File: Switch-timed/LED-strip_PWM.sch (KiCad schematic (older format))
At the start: 17 parts, among them IC1 MADW__ATTINY13-MM, P1 CONN_2, P2 CONN_2, T1 AO3400, U1 MCP6001, U2 MCP1804-SOT23-5

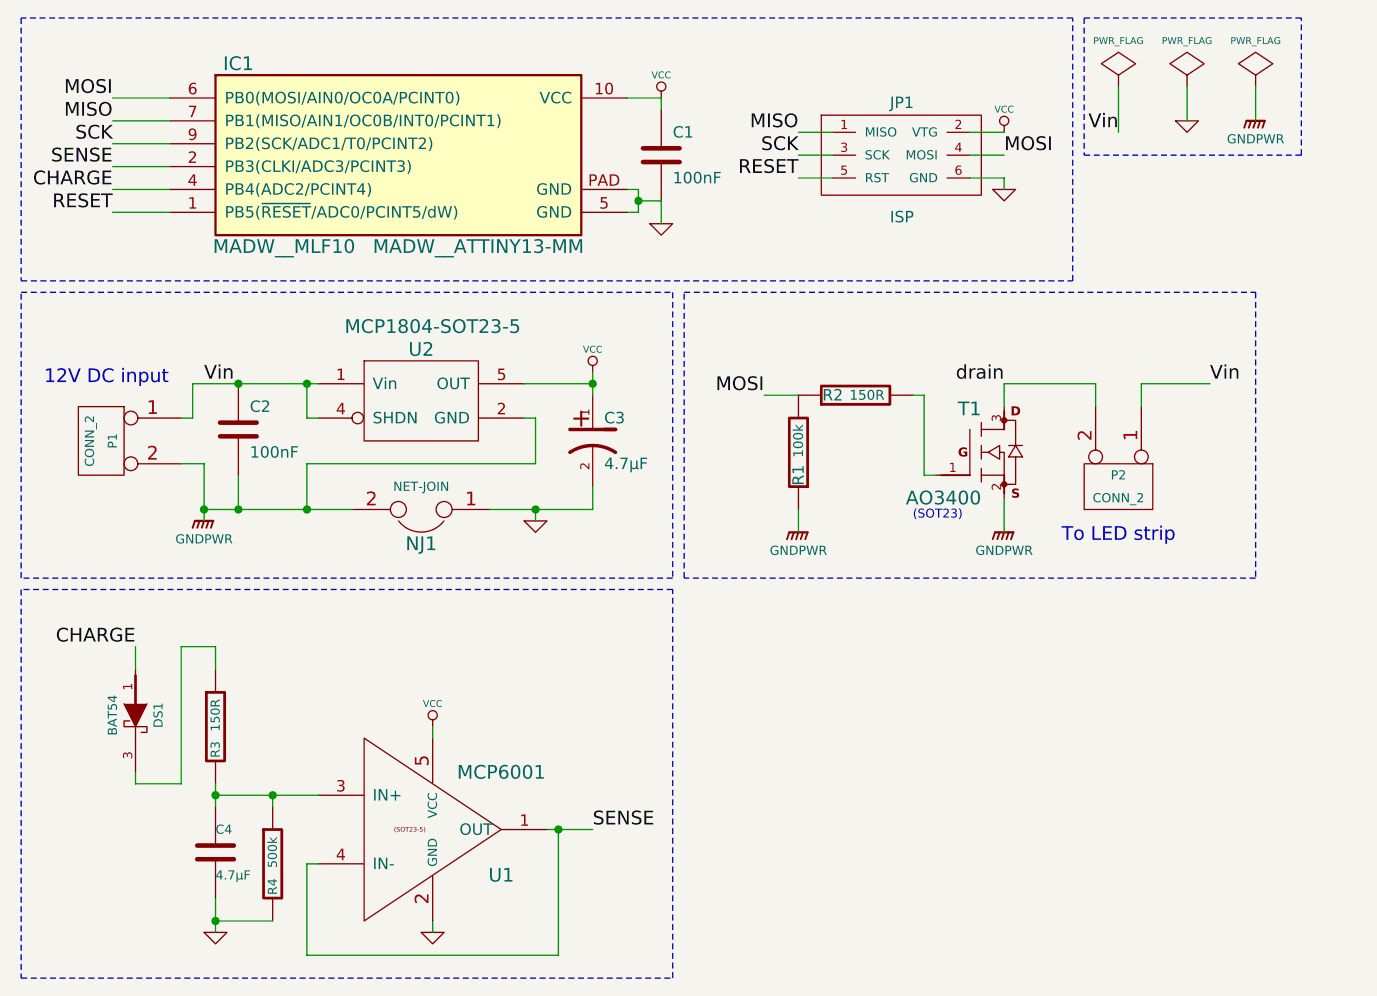
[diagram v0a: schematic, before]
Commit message: Switch-timed: switched to ATtiny10 SOT23-6.
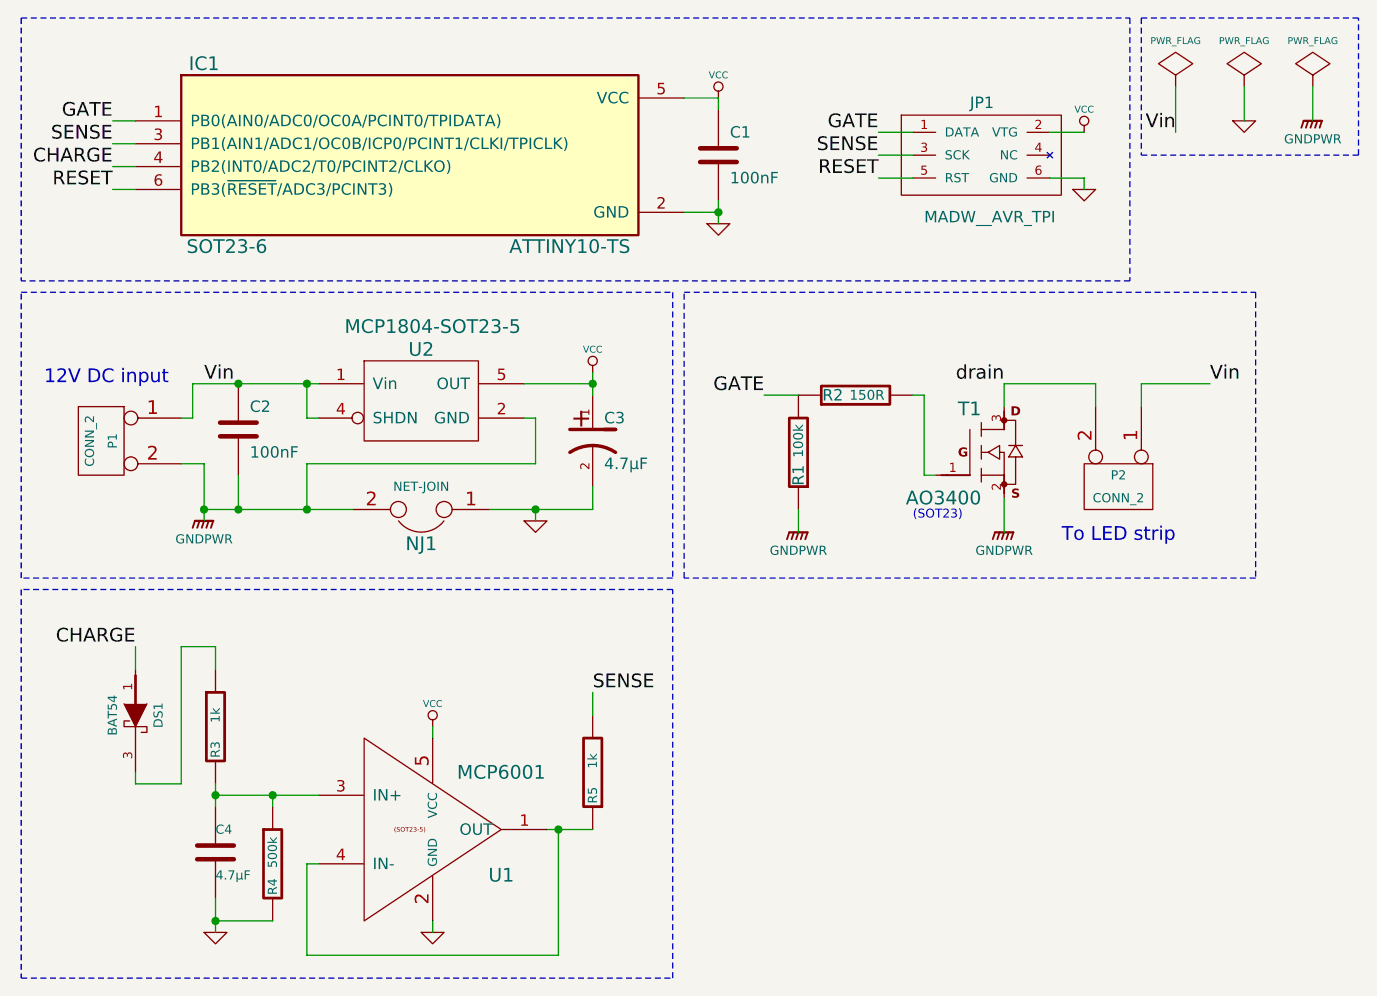
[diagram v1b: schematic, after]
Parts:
- removed IC1: MADW__ATTINY13-MM, MADW__MLF10, symbol MADW__ATTINY13-MM
- removed JP1: ISP, symbol MADW__AVR_ISP
- added IC1: ATTINY10-TS, SOT23-6, symbol ATTINY10-TS
- added JP1: MADW__AVR_TPI, symbol MADW__AVR_TPI
- added R5: 1k, symbol R
- R3: value 150R -> 1k
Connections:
- net CHARGE: now also IC1.4 (PB2(INT0/ADC2/T0/PCINT2/CLKO))
- net GND: now also IC1.2 (GND), JP1.6 (GND)
- net RESET: now also IC1.6 (PB3(~RESET~/ADC3/PCINT3)), JP1.5 (RST)
- net SENSE: now also IC1.3 (PB1(AIN1/ADC1/OC0B/ICP0/PCINT1/CLKI/TPICLK)), JP1.3 (SCK), R5.2; no longer U1.1 (OUT), U1.4 (IN-)
- net VCC: now also IC1.5 (VCC), JP1.2 (VTG)
- net MOSI renamed GATE
- net GATE: now also IC1.1 (PB0(AIN0/ADC0/OC0A/PCINT0/TPIDATA)), JP1.1 (DATA)
- new net: R5.1, U1.1 (OUT), U1.4 (IN-)
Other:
- moved on the sheet: C1

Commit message: Revert "Switch-timed: switched to ATtiny10 SOT23-6."
This reverts commit 7426c306dc58e77c9809db77e26f6b62b76c1d9c.

C + ATtiny10 not supported by avr-gcc
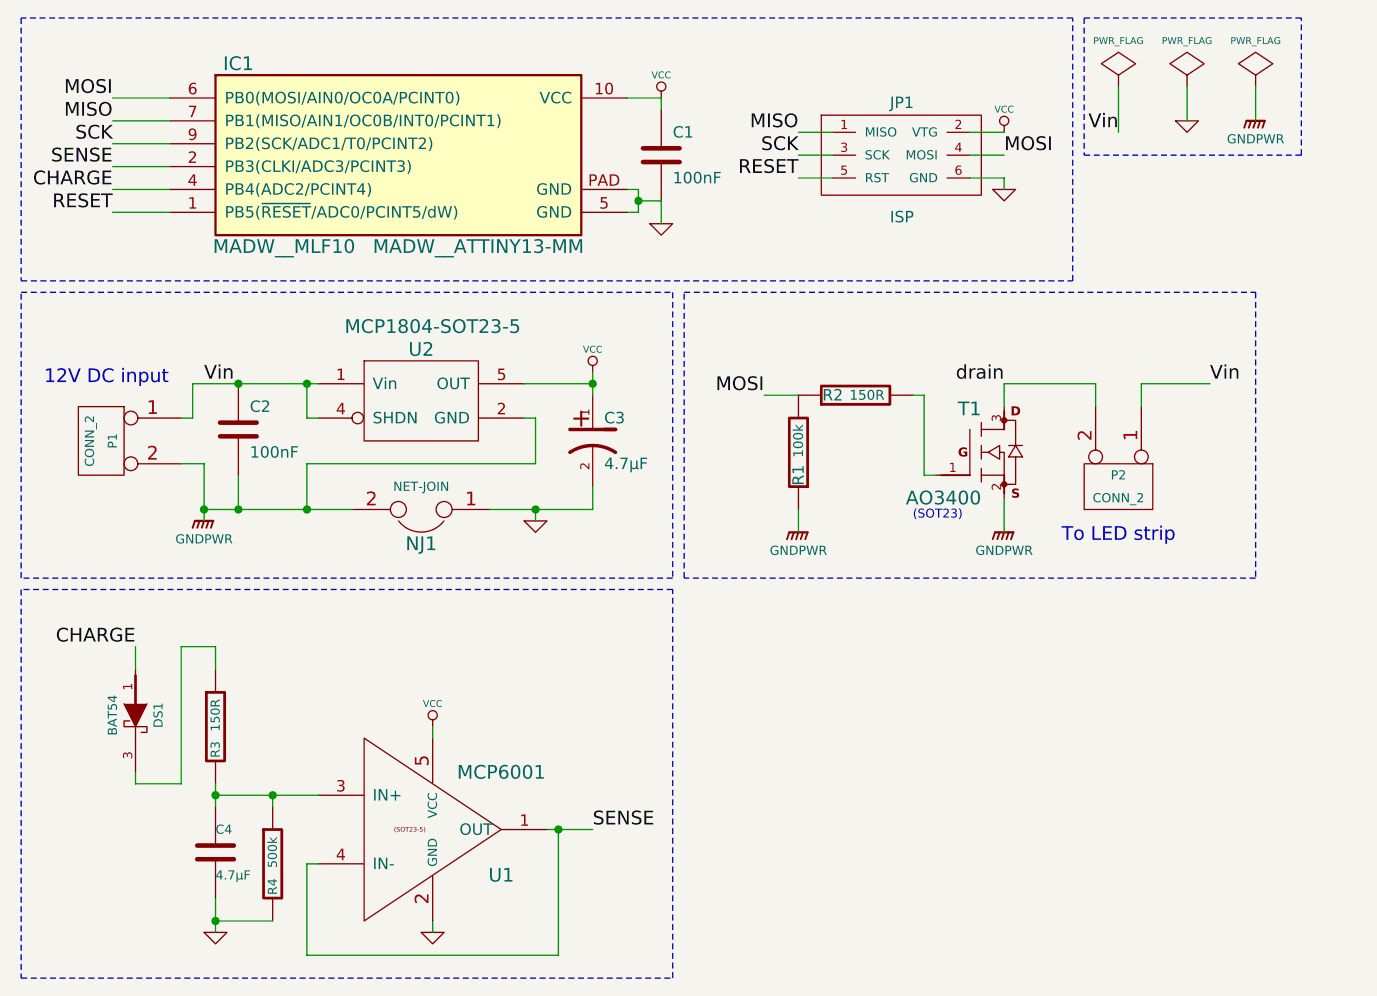
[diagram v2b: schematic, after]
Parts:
- removed IC1: ATTINY10-TS, SOT23-6, symbol ATTINY10-TS
- removed JP1: MADW__AVR_TPI, symbol MADW__AVR_TPI
- removed R5: 1k, symbol R
- added IC1: MADW__ATTINY13-MM, MADW__MLF10, symbol MADW__ATTINY13-MM
- added JP1: ISP, symbol MADW__AVR_ISP
- R3: value 1k -> 150R
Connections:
- net CHARGE: now also IC1.4 (PB4(ADC2/PCINT4))
- net GND: now also IC1.5 (GND), IC1.PAD (GND), JP1.6 (GND)
- net RESET: now also IC1.1 (PB5(~RESET~/ADC0/PCINT5/dW)), JP1.5 (RST)
- net SENSE: now also U1.1 (OUT), U1.4 (IN-), IC1.2 (PB3(CLKI/ADC3/PCINT3))
- net VCC: now also IC1.10 (VCC), JP1.2 (VTG)
- net GATE renamed MOSI
- net MOSI: now also IC1.6 (PB0(MOSI/AIN0/OC0A/PCINT0)), JP1.4 (MOSI)
- new net MISO: IC1.7 (PB1(MISO/AIN1/OC0B/INT0/PCINT1)), JP1.1 (MISO)
- new net SCK: IC1.9 (PB2(SCK/ADC1/T0/PCINT2)), JP1.3 (SCK)
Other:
- moved on the sheet: C1
